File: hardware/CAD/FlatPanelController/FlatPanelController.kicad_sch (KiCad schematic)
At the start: 24 parts, among them J1 Barrel_Jack_Switch_Pin3Ring, Q1 DMG3414U, Q2 DMG3414U, Q3 DMG3414U, Q4 DMG3414U, Q5 DMP3099L, SW1 SW_Push_LED, SW2 SW_Push_LED, SW3 SW_Push_LED, SW4 SW_Push_LED, U1 ESP32-WROOM-32E, U2 TSR1-2433E, U3 TSL25911FN, U4 LTR-303ALS-01, U5 MCP9804_MSOP, U6 AS1115-BSST, U7 LM4040CYM3-2.5, U8 CC04-41SURKWA

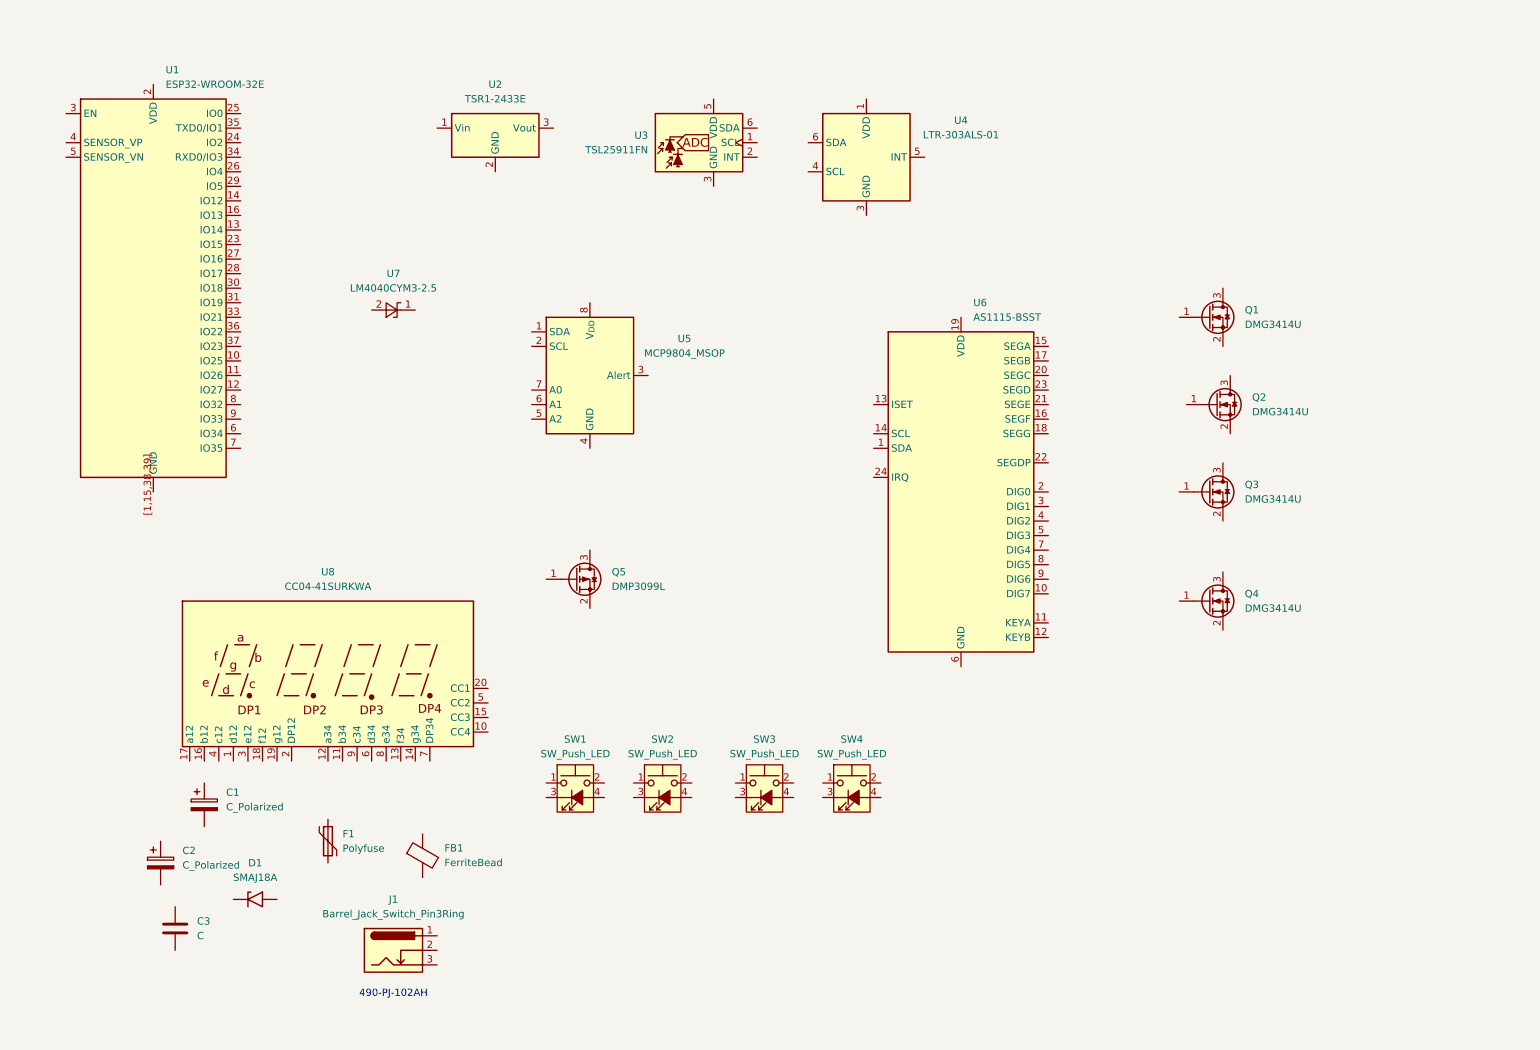
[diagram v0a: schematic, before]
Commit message: progress on design
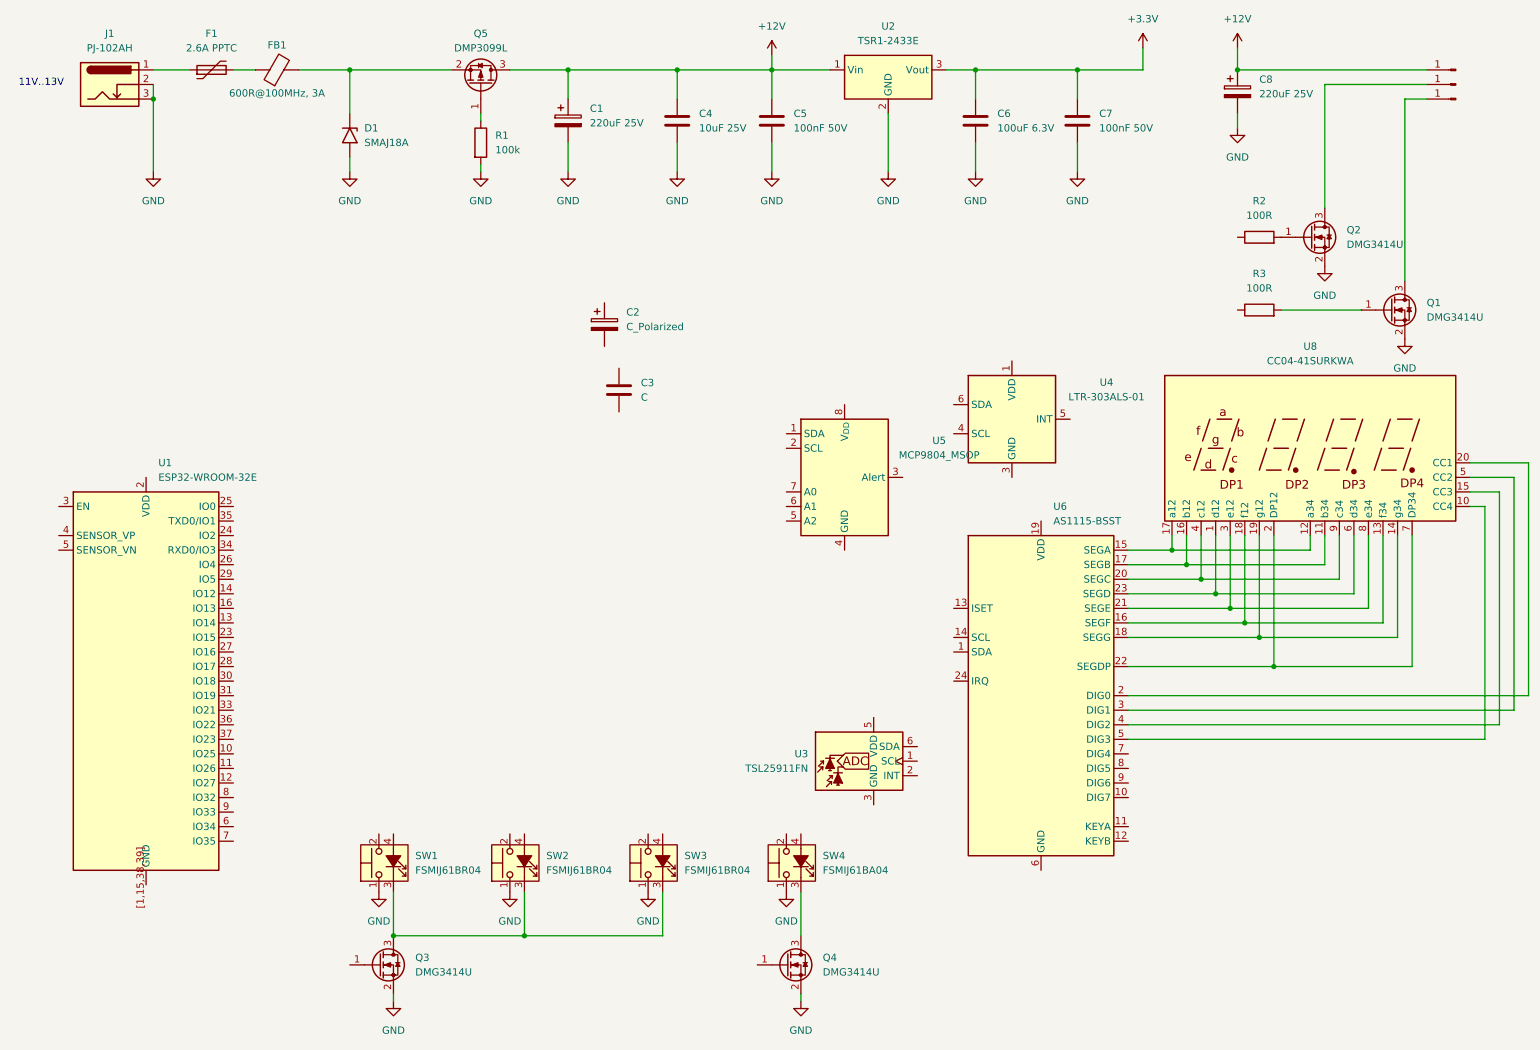
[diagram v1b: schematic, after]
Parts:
- removed U7: LM4040CYM3-2.5, Package_TO_SOT_SMD:SOT-23, symbol aa_MyParts:LM4040CYM3-2.5
- added C4: 10uF 25V, Capacitor_SMD:C_0805_2012Metric, symbol Device:C
- added C5, C7: 100nF 50V, Capacitor_SMD:C_0603_1608Metric, symbol Device:C
- added C6: 100uF 6.3V, Capacitor_SMD:C_1206_3216Metric, symbol Device:C
- added C8: 220uF 25V, Capacitor_THT:CP_Radial_D6.3mm_P2.50mm, symbol Device:C_Polarized
- added J2, J3, J4: Conn_01x01_Pin, TestPoint:TestPoint_Pad_4.0x4.0mm, symbol Connector:Conn_01x01_Pin
- added R1: 100k, symbol Device:R
- added R2, R3: 100R, symbol Device:R
- C1: value C_Polarized -> 220uF 25V; footprint (none) -> Capacitor_THT:CP_Radial_D6.3mm_P2.50mm
- F1: value Polyfuse -> 2.6A PPTC; footprint (none) -> Fuse:Fuse_1812_4532Metric
- FB1: value FerriteBead -> 600R@100MHz, 3A; footprint (none) -> Inductor_SMD:L_1210_3225Metric
- J1: value Barrel_Jack_Switch_Pin3Ring -> PJ-102AH; footprint (none) -> Connector_BarrelJack:BarrelJack_CUI_PJ-102AH_Horizontal
- SW1, SW2, SW3: value SW_Push_LED -> FSMIJ61BR04
- SW4: value SW_Push_LED -> FSMIJ61BA04
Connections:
- net GND: now reaches SW3.1
- net GND: now also C1.2, D1.2 (A2), J1.2, J1.3, Q1.2 (S), Q2.2 (S), Q3.2 (S), Q4.2 (S), SW1.1, SW2.1, SW4.1, U2.2 (GND), C4.2, C5.2, C6.2, C7.2, C8.2, R1.2
- net at SW3.3 (K): now also Q3.3 (D), SW1.3 (K), SW2.3 (K)
- net at Q1.1 (G): now also R3.2
- net at Q1.3 (D): now also J4.1 (Pin_1)
- net +12V: now reaches U2.1 (Vin)
- net +12V: now also C1.1, Q5.3 (D), C4.1, C5.1, C8.1, J2.1 (Pin_1)
- net +3.3V: now reaches U2.3 (Vout)
- net +3.3V: now also C6.1, C7.1
- net at U6.15 (SEGA): now also U8.12 (a34), U8.17 (a12)
- net at U6.16 (SEGF): now also U8.13 (f34), U8.18 (f12)
- net at U6.17 (SEGB): now also U8.11 (b34), U8.16 (b12)
- net at U6.18 (SEGG): now also U8.14 (g34), U8.19 (g12)
- net at U6.2 (DIG0): now also U8.20 (CC1)
- net at U6.20 (SEGC): now also U8.4 (c12), U8.9 (c34)
- net at U6.21 (SEGE): now also U8.3 (e12), U8.8 (e34)
- net at U6.22 (SEGDP): now also U8.2 (DP12), U8.7 (DP34)
- net at U6.23 (SEGD): now also U8.1 (d12), U8.6 (d34)
- net at U6.3 (DIG1): now also U8.5 (CC2)
- net at U6.4 (DIG2): now also U8.15 (CC3)
- net at U6.5 (DIG3): now also U8.10 (CC4)
- net at FB1.1: now also F1.2
- net at FB1.2: now also D1.1 (A1), Q5.2 (S)
- net at J1.1: now also F1.1
- net at Q4.3 (D): now also SW4.3 (K)
- net at Q5.1 (G): now also R1.1
- net at Q2.1 (G): now also R2.2
- net at Q2.3 (D): now also J3.1 (Pin_1)
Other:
- note added: "11V..13V"
- note removed: "490-PJ-102AH"
- moved on the sheet: C1, C2, C3, D1, F1, FB1, J1, Q1, Q2, Q3, Q4, SW1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
